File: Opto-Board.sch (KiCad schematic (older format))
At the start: 62 parts, among them J1 Screw_Terminal_01x08, J2 Screw_Terminal_01x08, J3 Screw_Terminal_01x08, J4 Screw_Terminal_01x02, U1 PC817, U2 PC817, U3 PC817, U4 PC817, U5 PC817, U6 PC817, U7 PC817, U8 PC817

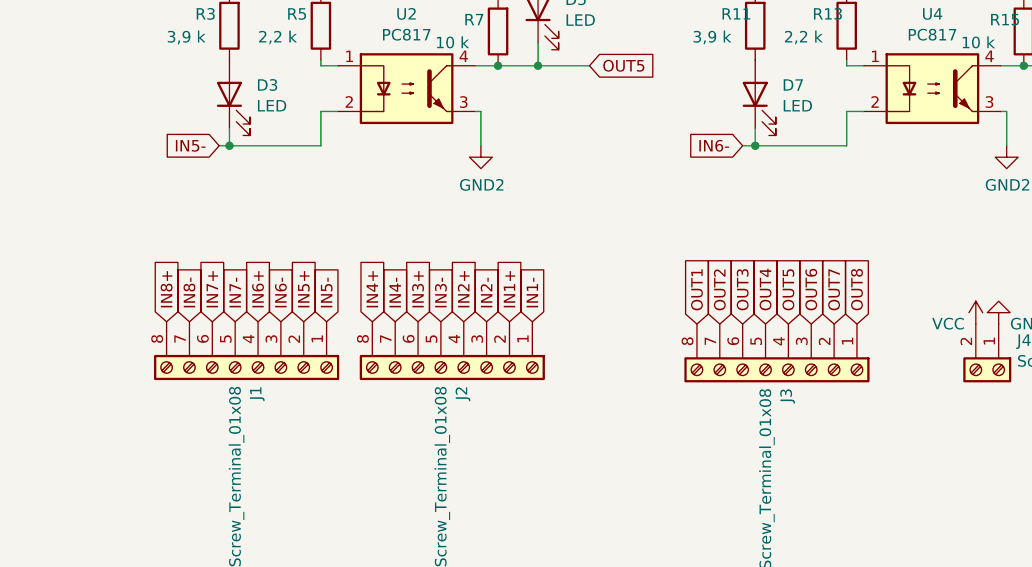
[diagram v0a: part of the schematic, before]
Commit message: Some fixes
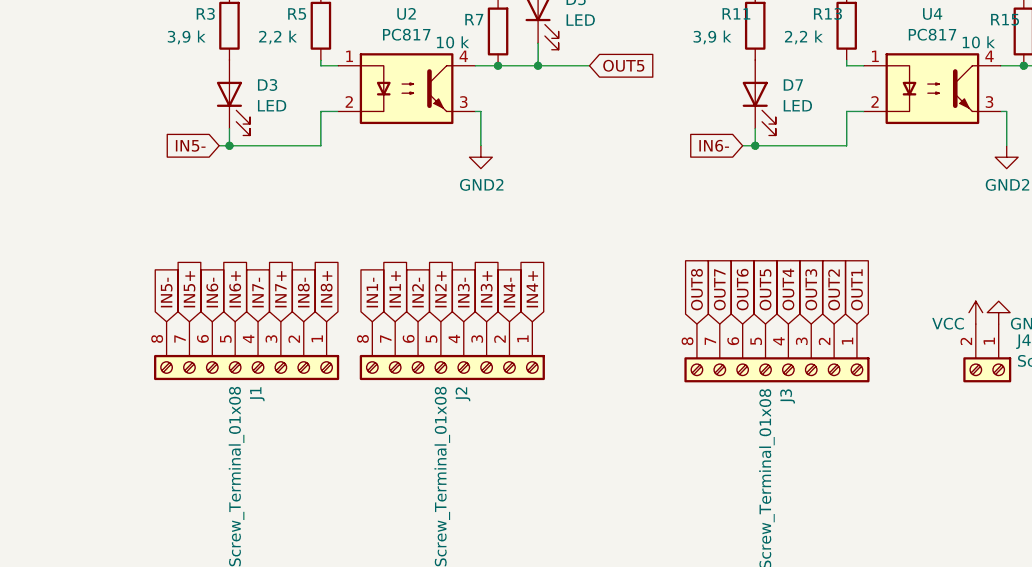
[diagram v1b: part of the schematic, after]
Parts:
- J1, J2, J3: footprint TerminalBlock_Phoenix:TerminalBlock_Phoenix_MKDS-3-8-5.08_1x08_P5.08mm_Horizontal -> TerminalBlock_Phoenix:TerminalBlock_Phoenix_MKDS-1,5-8_1x08_P5.00mm_Horizontal
- J4: footprint TerminalBlock_Phoenix:TerminalBlock_Phoenix_MKDS-3-2-5.08_1x02_P5.08mm_Horizontal -> TerminalBlock_Phoenix:TerminalBlock_Phoenix_MKDS-1,5-2_1x02_P5.00mm_Horizontal
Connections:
- net IN1+: now also J2.7 (Pin_7); no longer J2.2 (Pin_2)
- net IN1-: now also J2.8 (Pin_8); no longer J2.1 (Pin_1)
- net IN2+: now also J2.5 (Pin_5); no longer J2.4 (Pin_4)
- net IN2-: now also J2.6 (Pin_6); no longer J2.3 (Pin_3)
- net IN3+: now also J2.3 (Pin_3); no longer J2.6 (Pin_6)
- net IN3-: now also J2.4 (Pin_4); no longer J2.5 (Pin_5)
- net IN4+: now also J2.1 (Pin_1); no longer J2.8 (Pin_8)
- net IN4-: now also J2.2 (Pin_2); no longer J2.7 (Pin_7)
- net IN5+: now also J1.7 (Pin_7); no longer J1.2 (Pin_2)
- net IN5-: now also J1.8 (Pin_8); no longer J1.1 (Pin_1)
- net IN6+: now also J1.5 (Pin_5); no longer J1.4 (Pin_4)
- net IN6-: now also J1.6 (Pin_6); no longer J1.3 (Pin_3)
- net IN7+: now also J1.3 (Pin_3); no longer J1.6 (Pin_6)
- net IN7-: now also J1.4 (Pin_4); no longer J1.5 (Pin_5)
- net IN8+: now also J1.1 (Pin_1); no longer J1.8 (Pin_8)
- net IN8-: now also J1.2 (Pin_2); no longer J1.7 (Pin_7)
- net OUT1: now also J3.1 (Pin_1); no longer J3.8 (Pin_8)
- net OUT2: now also J3.2 (Pin_2); no longer J3.7 (Pin_7)
- net OUT3: now also J3.3 (Pin_3); no longer J3.6 (Pin_6)
- net OUT4: now also J3.4 (Pin_4); no longer J3.5 (Pin_5)
- net OUT5: now also J3.5 (Pin_5); no longer J3.4 (Pin_4)
- net OUT6: now also J3.6 (Pin_6); no longer J3.3 (Pin_3)
- net OUT7: now also J3.7 (Pin_7); no longer J3.2 (Pin_2)
- net OUT8: now also J3.8 (Pin_8); no longer J3.1 (Pin_1)
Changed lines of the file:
@@
 F 0 "J2" H 2680 4512 50  0000 L CNN
 F 1 "Screw_Terminal_01x08" H 2680 4421 50  0000 L CNN
-F 2 "TerminalBlock_Phoenix:TerminalBlock_Phoenix_MKDS-3-8-5.08_1x08_P5.08mm_Horizontal" H 2600 4520 50  0001 C CNN
+F 2 "TerminalBlock_Phoenix:TerminalBlock_Phoenix_MKDS-1,5-8_1x08_P5.00mm_Horizontal" H 2600 4520 50  0001 C CNN
 F 3 "~" H 2600 4520 50  0001 C CNN
 	1    2600 4520
@@
 F 0 "J3" H 4100 4522 50  0000 L CNN
 F 1 "Screw_Terminal_01x08" H 4100 4431 50  0000 L CNN
-F 2 "TerminalBlock_Phoenix:TerminalBlock_Phoenix_MKDS-3-8-5.08_1x08_P5.08mm_Horizontal" H 4020 4530 50  0001 C CNN
+F 2 "TerminalBlock_Phoenix:TerminalBlock_Phoenix_MKDS-1,5-8_1x08_P5.00mm_Horizontal" H 4020 4530 50  0001 C CNN
 F 3 "~" H 4020 4530 50  0001 C CNN
 	1    4020 4530
@@
 F 0 "J1" H 1780 4512 50  0000 L CNN
 F 1 "Screw_Terminal_01x08" H 1780 4421 50  0000 L CNN
-F 2 "TerminalBlock_Phoenix:TerminalBlock_Phoenix_MKDS-3-8-5.08_1x08_P5.08mm_Horizontal" H 1700 4520 50  0001 C CNN
+F 2 "TerminalBlock_Phoenix:TerminalBlock_Phoenix_MKDS-1,5-8_1x08_P5.00mm_Horizontal" H 1700 4520 50  0001 C CNN
 F 3 "~" H 1700 4520 50  0001 C CNN
 	1    1700 4520
@@
 Wire Wire Line
 	6175 3550 6575 3550
+Text GLabel 2300 4320 1    50   Input ~ 0
+IN1+
+Text GLabel 2200 4320 1    50   Input ~ 0
+IN1-
+Text GLabel 2500 4320 1    50   Input ~ 0
+IN2+
+Text GLabel 2400 4320 1    50   Input ~ 0
+IN2-
+Text GLabel 2700 4320 1    50   Input ~ 0
+IN3+
+Text GLabel 2600 4320 1    50   Input ~ 0
+IN3-
+Text GLabel 2900 4320 1    50   Input ~ 0
+IN4+
 Text GLabel 2800 4320 1    50   Input ~ 0
-IN1+
-Text GLabel 2900 4320 1    50   Input ~ 0
-IN1-
-Text GLabel 2600 4320 1    50   Input ~ 0
-IN2+
-Text GLabel 2700 4320 1    50   Input ~ 0
-IN2-
-Text GLabel 2400 4320 1    50   Input ~ 0
-IN3+
-Text GLabel 2500 4320 1    50   Input ~ 0
-IN3-
-Text GLabel 2200 4320 1    50   Input ~ 0
-IN4+
-Text GLabel 2300 4320 1    50   Input ~ 0
 IN4-
+Text GLabel 1400 4320 1    50   Input ~ 0
+IN5+
+Text GLabel 1300 4320 1    50   Input ~ 0
+IN5-
+Text GLabel 1600 4320 1    50   Input ~ 0
+IN6+
+Text GLabel 1500 4320 1    50   Input ~ 0
+IN6-
+Text GLabel 1800 4320 1    50   Input ~ 0
+IN7+
+Text GLabel 1700 4320 1    50   Input ~ 0
+IN7-
+Text GLabel 2000 4320 1    50   Input ~ 0
+IN8+
 Text GLabel 1900 4320 1    50   Input ~ 0
-IN5+
-Text GLabel 2000 4320 1    50   Input ~ 0
-IN5-
-Text GLabel 1700 4320 1    50   Input ~ 0
-IN6+
-Text GLabel 1800 4320 1    50   Input ~ 0
-IN6-
-Text GLabel 1500 4320 1    50   Input ~ 0
-IN7+
-Text GLabel 1600 4320 1    50   Input ~ 0
-IN7-
-Text GLabel 1300 4320 1    50   Input ~ 0
-IN8+
-Text GLabel 1400 4320 1    50   Input ~ 0
 IN8-
+Text GLabel 4320 4330 1    50   Input ~ 0
+OUT1
+Text GLabel 4220 4330 1    50   Input ~ 0
+OUT2
+Text GLabel 4120 4330 1    50   Input ~ 0
+OUT3
+Text GLabel 4020 4330 1    50   Input ~ 0
+OUT4
+Text GLabel 3920 4330 1    50   Input ~ 0
+OUT5
+Text GLabel 3820 4330 1    50   Input ~ 0
+OUT6
+Text GLabel 3720 4330 1    50   Input ~ 0
+OUT7
 Text GLabel 3620 4330 1    50   Input ~ 0
-OUT1
-Text GLabel 3720 4330 1    50   Input ~ 0
-OUT2
-Text GLabel 3820 4330 1    50   Input ~ 0
-OUT3
-Text GLabel 3920 4330 1    50   Input ~ 0
-OUT4
-Text GLabel 4020 4330 1    50   Input ~ 0
-OUT5
-Text GLabel 4120 4330 1    50   Input ~ 0
-OUT6
-Text GLabel 4220 4330 1    50   Input ~ 0
-OUT7
-Text GLabel 4320 4330 1    50   Input ~ 0
 OUT8
 $Comp
@@
 F 0 "J4" V 4812 4610 50  0000 L CNN
 F 1 "Screw_Terminal_01x02" V 4903 4610 50  0000 L CNN
-F 2 "TerminalBlock_Phoenix:TerminalBlock_Phoenix_MKDS-3-2-5.08_1x02_P5.08mm_Horizontal" H 4940 4530 50  0001 C CNN
+F 2 "TerminalBlock_Phoenix:TerminalBlock_Phoenix_MKDS-1,5-2_1x02_P5.00mm_Horizontal" H 4940 4530 50  0001 C CNN
 F 3 "~" H 4940 4530 50  0001 C CNN
 	1    4940 4530
